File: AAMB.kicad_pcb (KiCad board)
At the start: 2 copper layers, 188 parts, among them J1 Screw_Terminal_01x04, J2 PJRAS4X2U01X, J3 SPKR L, J4 SPKR R, J5 Screw_Terminal_01x03, J6 Screw_Terminal_01x03, J7 Screw_Terminal_01x04, K1 G5LE-1, K2 G5LE-1, Q1 BC546, Q2 BC556, Q201 BC546, Q202 BC546, Q203 BC546, Q204 BD140, Q205 BD139, Q206 BD140, Q207 MJL21193, Q208 MJL21194, Q209 BC546, Q3 BC546, Q301 BC546, Q302 BC546, Q303 BC546, Q304 BD140, Q305 BD139, Q306 BD140, Q307 MJL21193, Q308 MJL21194, Q309 BC546, Q4 BD140, U1 TL072, U2 NE5532, U3 NE5532, U4 THAT2180, U5 DG509BEQ-T1-E3, U6 CD4071B

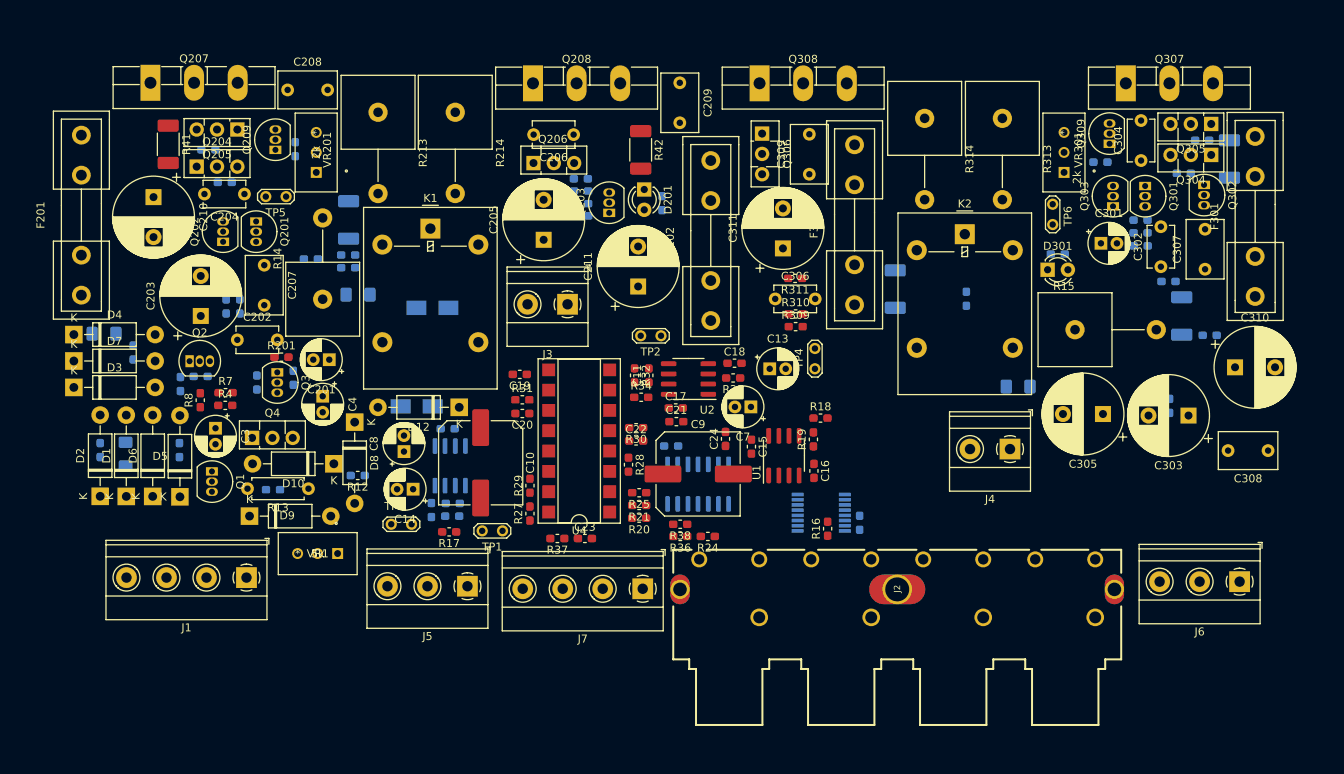
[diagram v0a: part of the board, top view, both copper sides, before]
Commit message: First pass auto-route
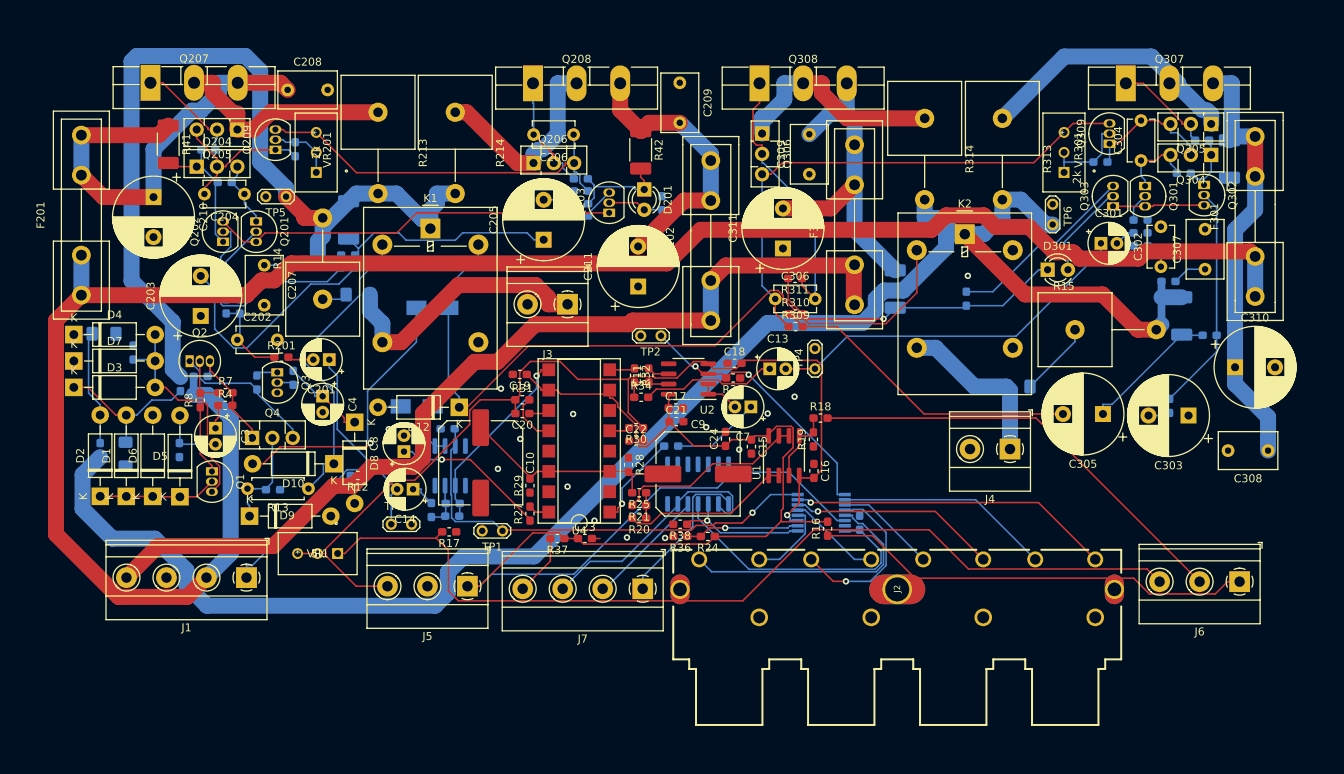
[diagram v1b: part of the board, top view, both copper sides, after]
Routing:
- net +35V: track 0.00 -> 247.4 mm
- net /pwr_audio_R: track 0.00 -> 206.4 mm
- net +12V: track 0.00 -> 165.5 mm
- net -12V: track 0.00 -> 125.2 mm, vias 0 -> 1
- net -35V: track 0.00 -> 118.3 mm
- net /volume/vol_pot_3: track 0.00 -> 117.2 mm
- net /pwr_audio_L: track 0.00 -> 110.9 mm
- net /short_protection_muting/RLY_-L_+R: track 0.00 -> 94.9 mm
- net Net-(C306-Pad1): track 0.00 -> 66.5 mm
- net /pre_vol_audio_L: track 0.00 -> 57.2 mm, vias 0 -> 1
- net /volume/vol_pot_1: track 0.00 -> 55.1 mm
- net /volume/vol_pot_2: track 0.00 -> 55.0 mm
- net /audio_pwr_R/P35_fused_R: track 0.00 -> 54.5 mm
- net /audio_pwr_L/P35_fused_L: track 0.00 -> 53.8 mm
- net Net-(Q201-Pad3): track 0.00 -> 50.8 mm
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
